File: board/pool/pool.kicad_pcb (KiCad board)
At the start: 2 copper layers, 65 x 30 mm, 54 parts, among them J1 -0.3, J2 ORP, J4 Raspberry_Pi_4, J5 Screw_Terminal_01x04, U1 TLV2372, U2 TLV2372, U3 TLV75801PDBV, U4 ADS1015IDGS, U5 MAX481E, U6 AP62300WU, U7 ISO1541

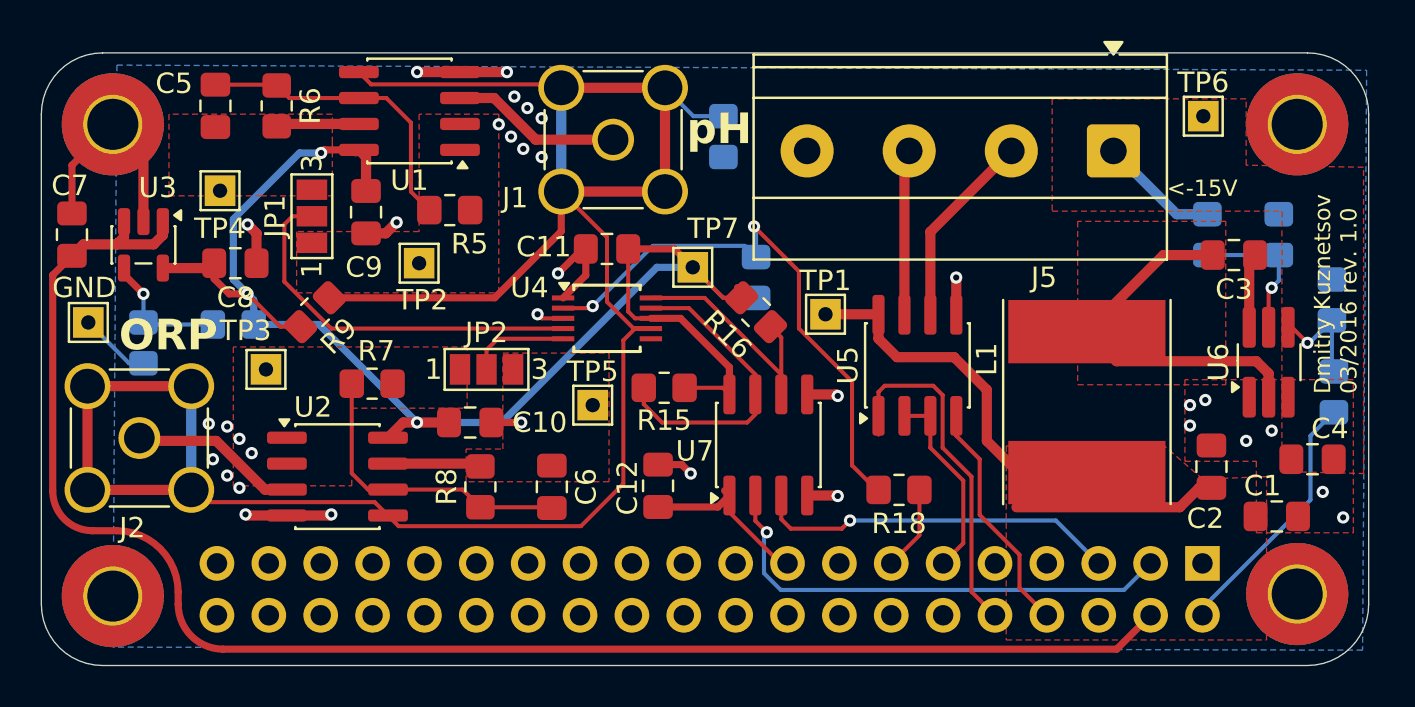
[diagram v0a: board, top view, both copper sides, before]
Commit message: Added rev 1.1 of the board
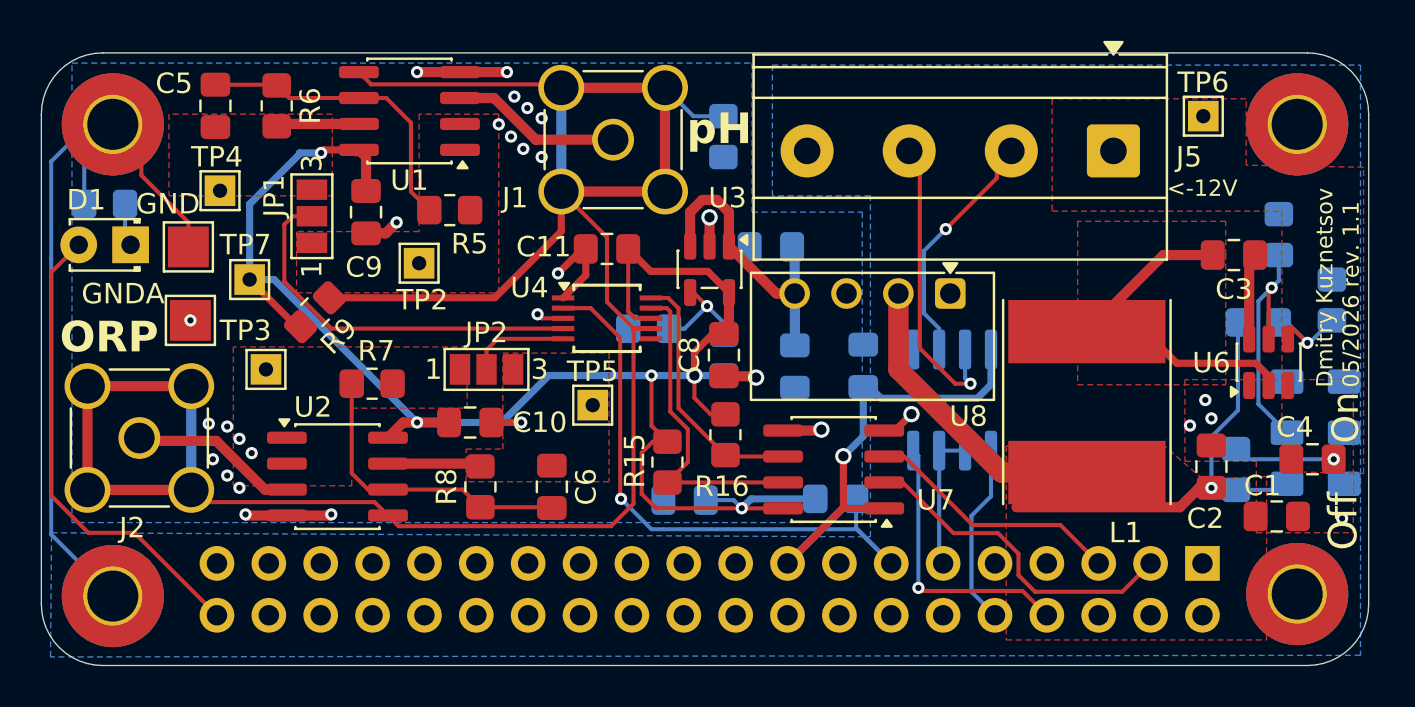
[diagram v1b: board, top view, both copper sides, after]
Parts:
- removed R18: 0, Resistor_SMD:R_0805_2012Metric_Pad1.20x1.40mm_HandSolder
- removed TP1: TestPoint, TestPoint:TestPoint_THTPad_1.5x1.5mm_Drill0.7mm
- removed TP8: GND, TestPoint:TestPoint_THTPad_1.5x1.5mm_Drill0.7mm
- added C13: 100n, Capacitor_SMD:C_0805_2012Metric_Pad1.18x1.45mm_HandSolder, B.Cu at (141.2, 91.8)
- added C14: 10u, Capacitor_SMD:C_0805_2012Metric_Pad1.18x1.45mm_HandSolder, B.Cu at (146.6, 85.3)
- added D1: LED, LED_THT:LED_D1.8mm_W3.3mm_H2.4mm, F.Cu at (114.0, 79.3)
- added GND: TestPoint, TestPoint:TestPoint_Pad_2.0x2.0mm, F.Cu at (116.8, 79.5)
- added GNDA: GNDA, TestPoint:TestPoint_Pad_2.0x2.0mm, F.Cu at (117.0, 83.0)
- added R13: 13k, Resistor_SMD:R_0805_2012Metric_Pad1.20x1.40mm_HandSolder, B.Cu at (112.8, 77.3)
- added SW1: SW_Slide_DPDT, mylib:CL-SB-22A, B.Cu at (177.6, 88.5)
- added U8: TEA1-0505, Converter_DCDC:Converter_DCDC_TRACO_TEA1-xxxx_THT, F.Cu at (154.2, 81.7)
- C12, C7, U5: moved to B.Cu
- TP7: value TestPoint -> GNDA
- U6: footprint Package_TO_SOT_SMD:TSOT-23-6_HandSoldering -> Package_TO_SOT_SMD:TSOT-23-6
- moved C7 34.2 mm to (145.4, 79.5), turned to 180 degrees
- moved U3 27.7 mm to (142.4, 80.5)
- moved R12 24.7 mm to (139.4, 83.5), turned to 0 degrees
- moved C8 24.3 mm to (143.1, 84.8), turned to 90 degrees
- moved R11 24.1 mm to (143.1, 84.8), turned to -90 degrees
- moved TP7 21.7 mm to (119.8, 81.0)
- moved C12 11.6 mm to (149.9, 85.3)
- moved R1 11.6 mm to (168.2, 90.3)
- moved R17 11.5 mm to (148.6, 91.8), turned to 0 degrees
- moved R16 6.18 mm to (143.2, 88.7), turned to -90 degrees
- moved R4 5.02 mm to (169.2, 83.2), turned to 0 degrees
- moved R15 3.64 mm to (140.3, 90.0), turned to -90 degrees
- moved U7 3.42 mm to (148.4, 90.3), turned to 180 degrees
- moved U5 2.40 mm to (154.2, 87.0)
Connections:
- C10 pad 2: GND -> GNDA
- C11 pad 2: GND -> GNDA
- C12 pad 1: Net-(U7-VCC1) -> +3V3
- C7 pad 1: +5V -> +5VA
- C7 pad 2: GND -> GNDA
- C8 pad 1: GND -> GNDA
- C9 pad 2: GND -> GNDA
- J4 pad 1: Net-(U7-VCC1) -> +3V3
- J4 pad 17: Net-(U7-VCC1) -> +3V3
- J4 pad 40: unconnected-(J4-GPIO21/SPI1_SCLK/PCM_DOUT-Pad40) -> Net-(D1-A)
- R1 pad 2: Net-(U6-EN) -> Net-(R1-Pad2)
- R10 pad 1: GND -> GNDA
- R12 pad 1: GND -> GNDA
- R17 pad 2: RDY_A -> RDY
- U1 pad 4: GND -> GNDA
- U2 pad 4: GND -> GNDA
- U3 pad 1: +5V -> +5VA
- U3 pad 2: GND -> GNDA
- U3 pad 3: +5V -> +5VA
- U4 pad 1: GND -> GNDA
- U4 pad 2: RDY_A -> RDY
- U4 pad 3: GND -> GNDA
- U5 pad 8: +5V -> +3V3
- U7 pad 1: Net-(U7-VCC1) -> +3V3
- U7 pad 5: GND -> GNDA
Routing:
- net +5V: track 119.8 -> 38.9 mm, vias 0 -> 1
- net RDY_A: track 28.0 -> 0.00 mm, vias 2 -> 0
- net RDY: track 4.17 -> 29.9 mm, vias 0 -> 1
- net +3V3: track 0.00 -> 24.8 mm, vias 0 -> 1
- net Net-(D1-A): track 0.00 -> 23.4 mm
- net GNDA: track 0.00 -> 22.8 mm, vias 0 -> 26
- net +5VA: track 0.00 -> 15.0 mm
- net Net-(U7-VCC1): track 8.77 -> 0.00 mm
- net Net-(J4-GPIO15/UART_RXD): track 17.4 -> 8.94 mm
- net /digital/SDA: track 23.9 -> 16.5 mm, vias 1 -> 0
- net VDDA: track 77.8 -> 84.6 mm, vias 3 -> 5
- net Net-(J5-Pin_3): track 8.45 -> 14.9 mm, vias 0 -> 1
- net /digital/SCL: track 17.9 -> 12.7 mm, vias 1 -> 0
- net Net-(U6-EN): track 7.25 -> 12.4 mm
- net Net-(J4-GPIO17/SPI1_~{CE1}): track 9.57 -> 6.88 mm
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- added copper zone on B.Cu, net GNDA
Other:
- board text added: "<-12V"
- board text added: "Dmitry Kuznetsov 05/2026 rev. 1.1"
- board text added: "Off"
- board text added: "On"
- board text removed: "<-15V"
- board text removed: "Dmitry Kuznetsov 03/2016 rev. 1.0"
